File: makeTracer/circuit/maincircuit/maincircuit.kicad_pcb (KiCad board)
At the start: 2 copper layers, 100 x 70 mm, 74 parts, among them IC1 PIC16F1778-I/SP, J1 PICKit3, J2 Sensor, J3 I^{2}C, J5 Motor_L, J6 Motor_R, P1 FrontsidePort, Q1 MP4212, Q2 MP4212, SW1 SW_DPDT_x2, SW2 Reset, SW3 Red, SW4 Green, U1 74HC00, U2 74HC595, U3 74HC595

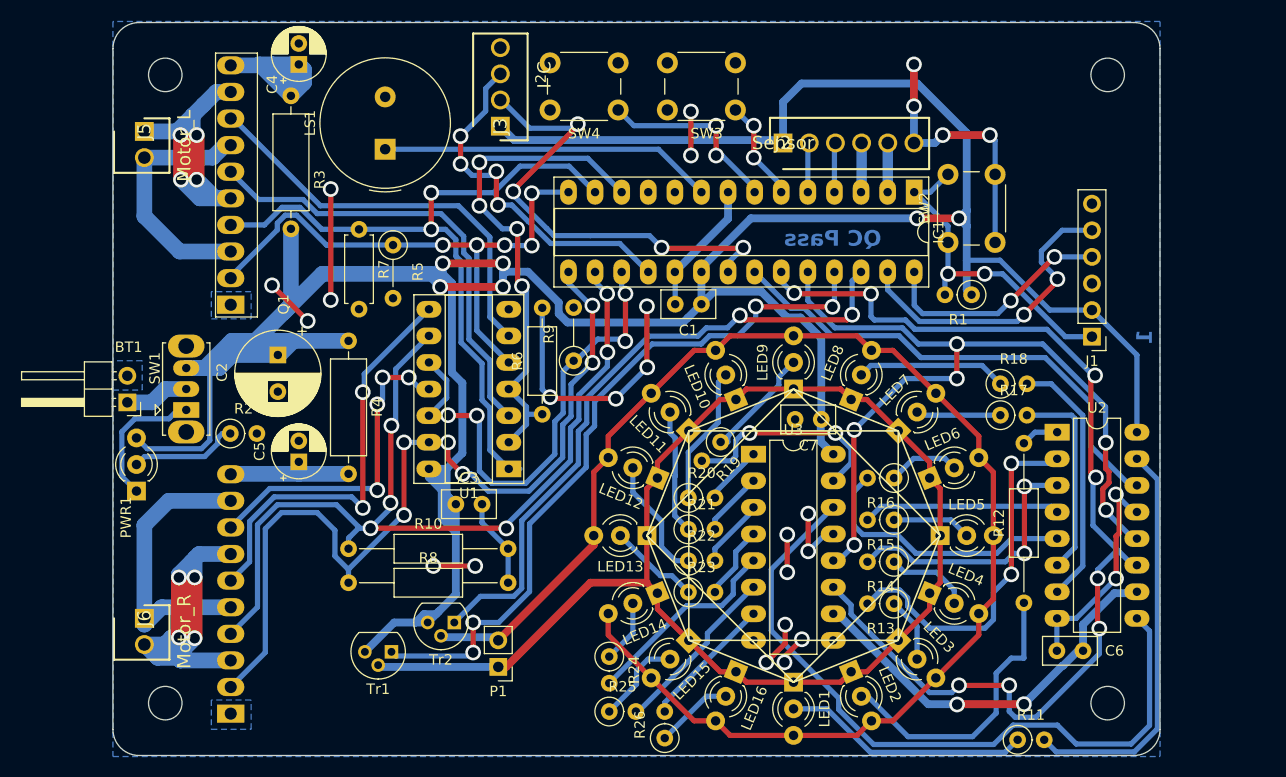
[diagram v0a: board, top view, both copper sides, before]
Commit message: fix: yabai jumper
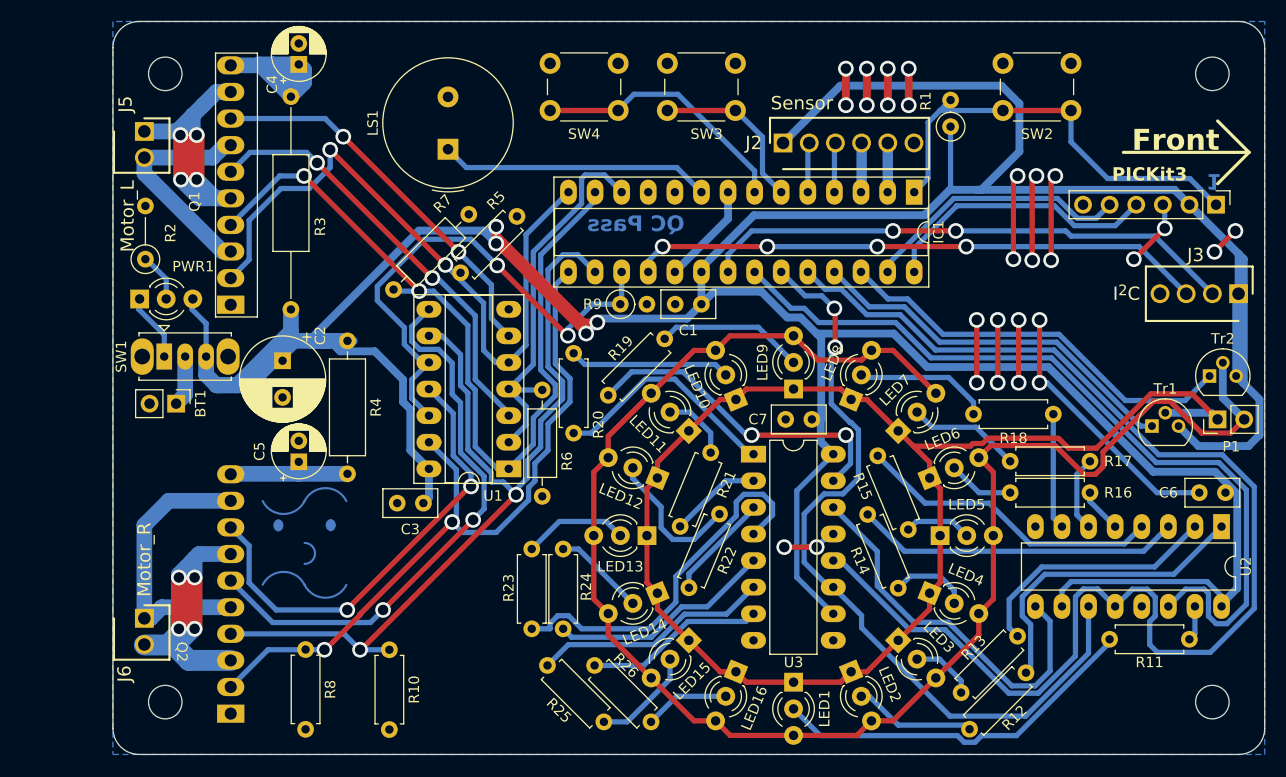
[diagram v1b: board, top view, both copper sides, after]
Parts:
- added REF**: KiCad-Logo2_8mm_SilkScreen, Symbol:KiCad-Logo2_8mm_SilkScreen, B.Cu at (52.0, 78.9)
- BT1: footprint Connector_PinHeader_2.54mm:PinHeader_1x02_P2.54mm_Horizontal -> Connector_PinHeader_2.54mm:PinHeader_1x02_P2.54mm_Vertical
- R10, R12, R8: footprint Resistor_THT:R_Axial_DIN0207_L6.3mm_D2.5mm_P15.24mm_Horizontal -> Resistor_THT:R_Axial_DIN0207_L6.3mm_D2.5mm_P7.62mm_Horizontal
- R11, R13, R14, R15, R16, R17, R18, R19, R20, R21, R22, R23, R24, R25, R26: footprint Resistor_THT:R_Axial_DIN0207_L6.3mm_D2.5mm_P2.54mm_Vertical -> Resistor_THT:R_Axial_DIN0207_L6.3mm_D2.5mm_P7.62mm_Horizontal
- R2: footprint Resistor_THT:R_Axial_DIN0207_L6.3mm_D2.5mm_P2.54mm_Vertical -> Resistor_THT:R_Axial_DIN0207_L6.3mm_D2.5mm_P5.08mm_Vertical
- R3: footprint Resistor_THT:R_Axial_DIN0309_L9.0mm_D3.2mm_P12.70mm_Horizontal -> Resistor_THT:R_Axial_DIN0309_L9.0mm_D3.2mm_P20.32mm_Horizontal
- R5: footprint Resistor_THT:R_Axial_DIN0207_L6.3mm_D2.5mm_P5.08mm_Vertical -> Resistor_THT:R_Axial_DIN0207_L6.3mm_D2.5mm_P7.62mm_Horizontal
- R7: footprint Resistor_THT:R_Axial_DIN0207_L6.3mm_D2.5mm_P7.62mm_Horizontal -> Resistor_THT:R_Axial_DIN0207_L6.3mm_D2.5mm_P10.16mm_Horizontal
- R9: footprint Resistor_THT:R_Axial_DIN0207_L6.3mm_D2.5mm_P5.08mm_Vertical -> Resistor_THT:R_Axial_DIN0207_L6.3mm_D2.5mm_P2.54mm_Vertical
- moved Tr2 75.9 mm to (124.7, 53.8), turned to 0 degrees
- moved Tr1 75.8 mm to (119.2, 58.5), turned to 0 degrees
- moved P1 72.7 mm to (125.5, 57.9), turned to 90 degrees
- moved J3 72.3 mm to (127.5, 45.9), turned to 180 degrees
- moved C6 20.3 mm to (126.2, 64.9)
- moved R2 18.5 mm to (23.1, 42.6), turned to 90 degrees
- moved PWR1 18.4 mm to (22.6, 46.4), turned to 0 degrees
- moved U2 18.1 mm to (125.9, 68.1), turned to -90 degrees
- moved R20 17.6 mm to (64.0, 51.6), turned to -90 degrees
- moved J1 17.3 mm to (125.3, 37.4), turned to -90 degrees
- moved R1 16.2 mm to (100.0, 29.9), turned to 90 degrees
- moved R23 15.5 mm to (60.0, 70.3), turned to -90 degrees
- moved R12 13.1 mm to (101.8, 87.5), turned to 45 degrees
- moved R11 13.0 mm to (115.2, 78.9)
- moved R19 11.2 mm to (72.7, 50.2)
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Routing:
- net /16x2LEDs/Flash: track 78.7 -> 124.7 mm, vias 6 -> 0
- net /16x2LEDs/LED1: track 38.8 -> 3.36 mm
- net /16x2LEDs/Select_Red: track 69.3 -> 36.8 mm, vias 4 -> 0
- net Net-(U2-QH'): track 68.5 -> 37.0 mm
- net /16x2LEDs/Data: track 47.4 -> 78.0 mm
- net GND: track 135.4 -> 106.5 mm, vias 26 -> 28
- net /16x2LEDs/LED13: track 7.10 -> 35.9 mm
- net /16x2LEDs/LED2: track 3.61 -> 29.6 mm
- net /16x2LEDs/Clock: track 102.8 -> 77.1 mm, vias 8 -> 2
- net /16x2LEDs/Select_Green: track 62.0 -> 39.9 mm, vias 2 -> 0
- net /16x2LEDs/LED6: track 26.2 -> 4.24 mm
- net I^{2}C_SCL: track 34.5 -> 54.9 mm
- net /16x2LEDs/Green_Src: track 138.3 -> 158.6 mm
- net /16x2LEDs/LED10: track 5.70 -> 22.3 mm
- net Net-(LED2-K): track 27.7 -> 11.6 mm
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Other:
- board size 100 x 70 mm -> 110 x 70 mm
- board text added: "Front"
- board text added: "PICKit3 Size"

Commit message: ohsaycanyouwip
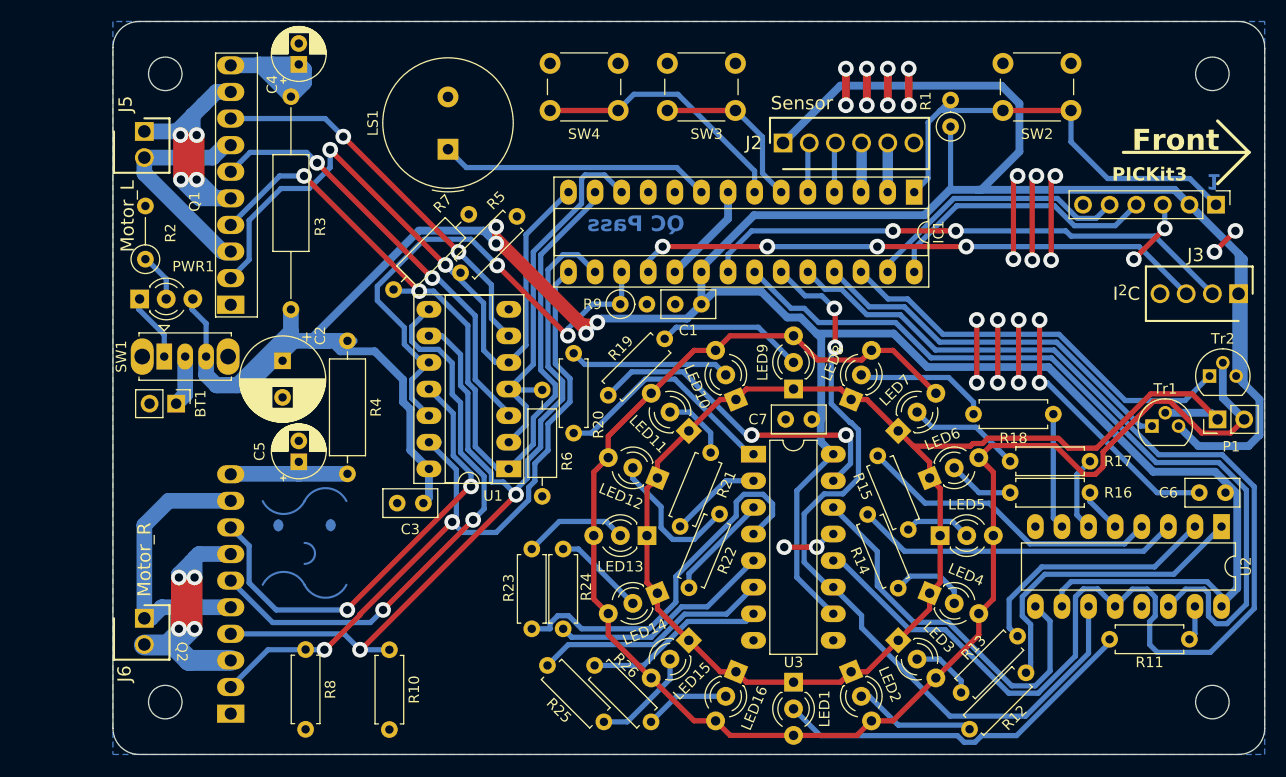
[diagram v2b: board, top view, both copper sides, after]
